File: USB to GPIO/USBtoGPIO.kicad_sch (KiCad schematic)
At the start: 3 parts, among them U1 STM32F030F4Px, U2 74HC595, U3 74HC165

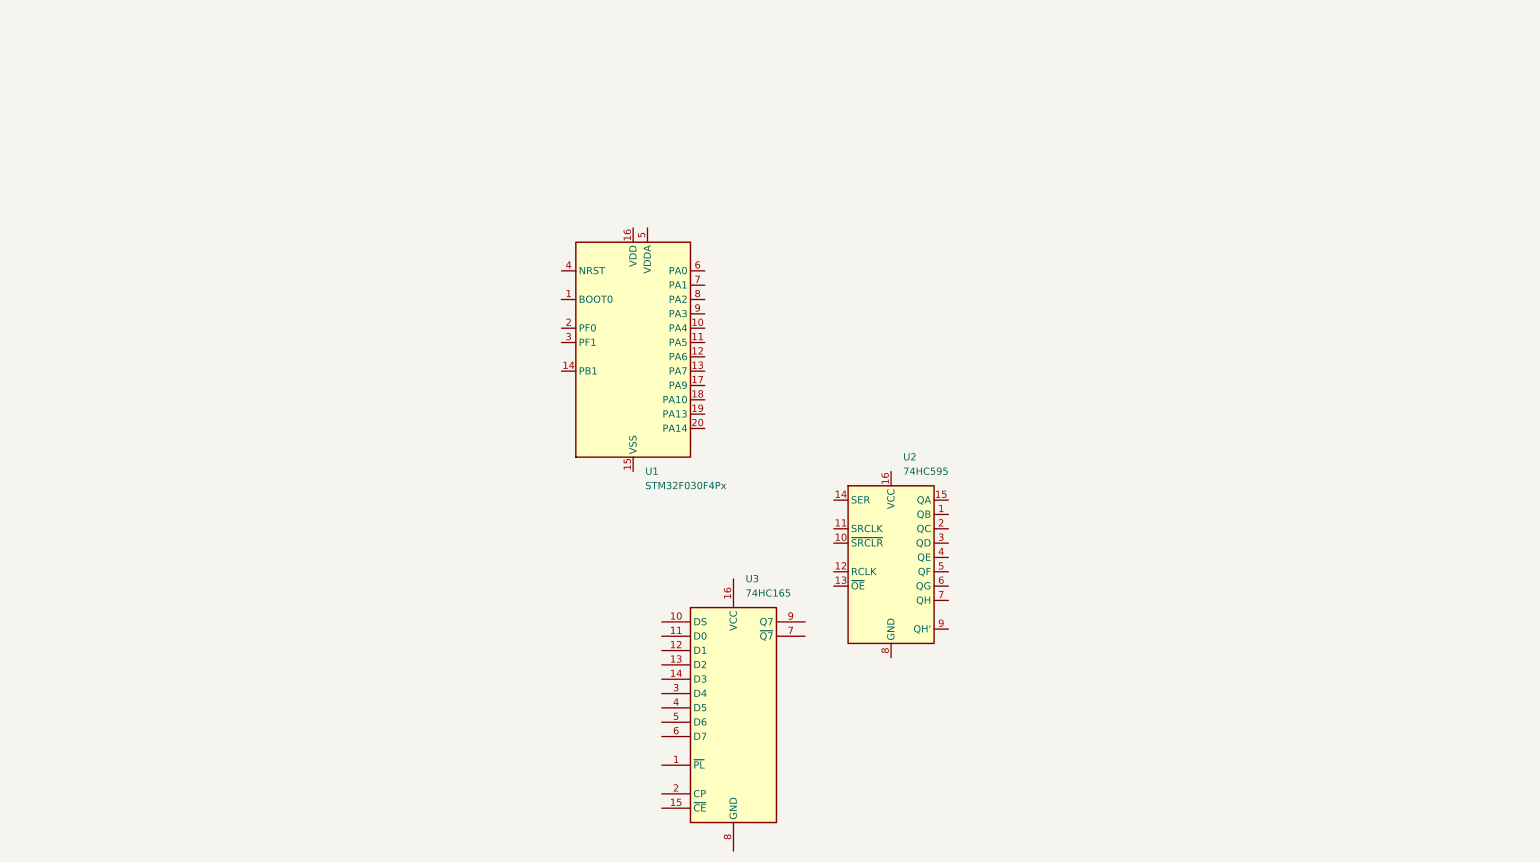
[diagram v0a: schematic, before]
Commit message: refresh
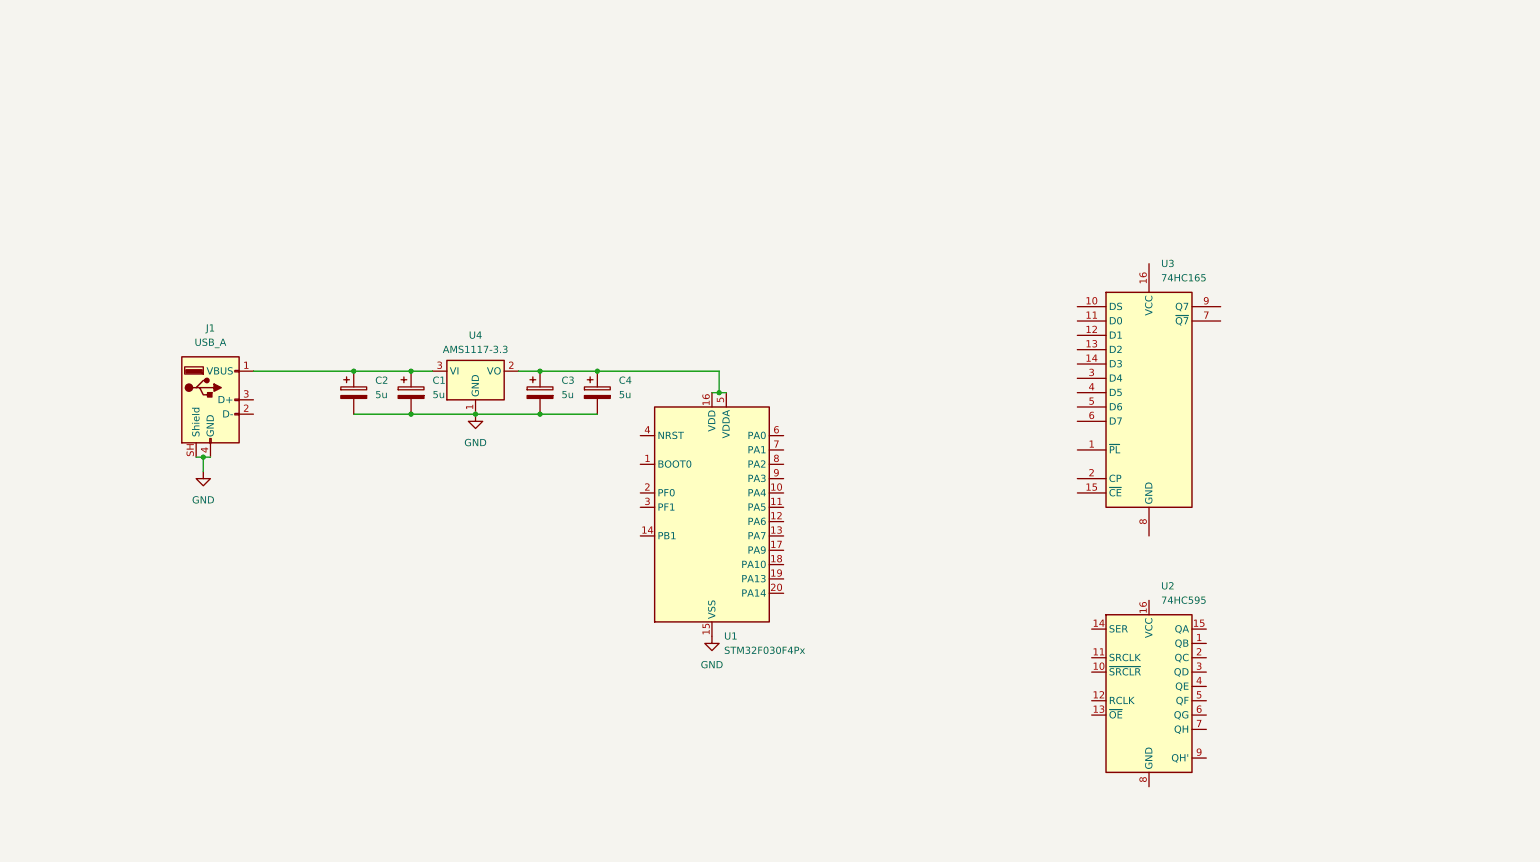
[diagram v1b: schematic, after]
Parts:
- added C1, C2, C3, C4: 5u, symbol Device:C_Polarized
- added J1: USB_A, Connector_USB:USB_A_TE_292303-7_Horizontal, symbol Connector:USB_A
- added U4: AMS1117-3.3, Package_TO_SOT_SMD:SOT-223-3_TabPin2, symbol Regulator_Linear:AMS1117-3.3
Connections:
- net GND: now reaches U1.15 (VSS)
- net GND: now also C1.2, C2.2, C3.2, C4.2, J1.4 (GND), J1.SH (Shield), U4.1 (GND)
- net at U1.16 (VDD): now also U1.5 (VDDA), C3.1, C4.1, U4.2 (VO)
- new net: C1.1, C2.1, J1.1 (VBUS), U4.3 (VI)
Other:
- moved on the sheet: U1, U2, U3

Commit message: refresh
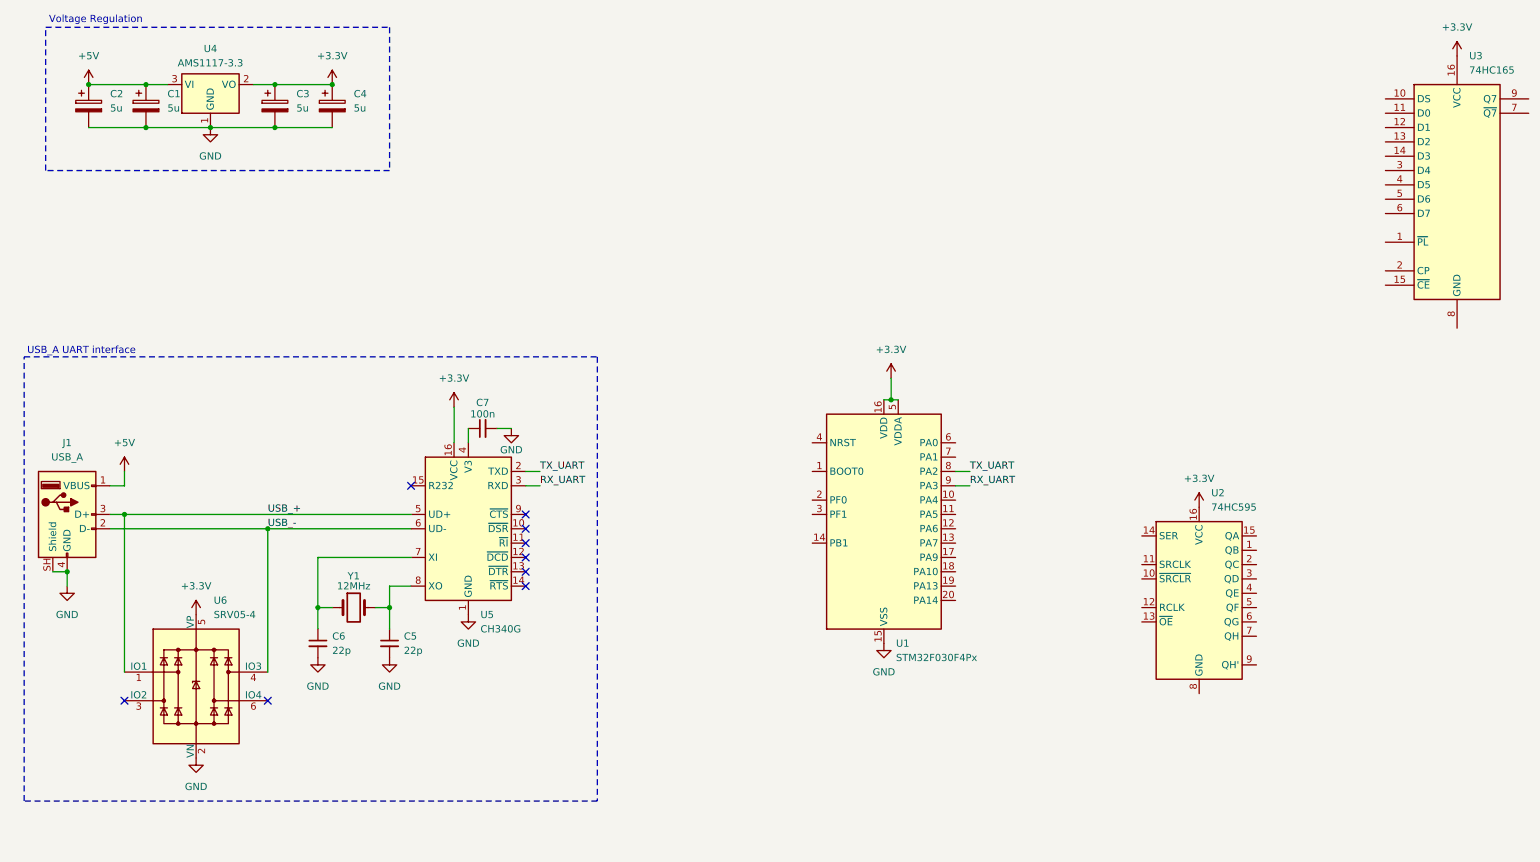
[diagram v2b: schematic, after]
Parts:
- added C5, C6: 22p, symbol Device:C_Small
- added C7: 100n, symbol Device:C_Small
- added U5: CH340G, Package_SO:SOIC-16_3.9x9.9mm_P1.27mm, symbol Interface_USB:CH340G
- added U6: SRV05-4, Package_TO_SOT_SMD:SOT-23-6, symbol Power_Protection:SRV05-4
- added Y1: 12MHz, symbol Device:Crystal
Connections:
- net GND: now also C5.2, C6.2, C7.2, U5.1 (GND), U6.2 (VN)
- net +5V: now reaches C1.1, C2.1, J1.1 (VBUS), U4.3 (VI)
- net +3.3V: now reaches C3.1, C4.1, U1.16 (VDD), U1.5 (VDDA), U4.2 (VO)
- net +3.3V: now also U2.16 (VCC), U3.16 (VCC), U5.16 (VCC), U6.5 (VP)
- net TX_UART: now reaches U1.8 (PA2)
- net TX_UART: now also U5.2 (TXD)
- net RX_UART: now reaches U1.9 (PA3)
- net RX_UART: now also U5.3 (RXD)
- net USB_-: now reaches J1.2 (D-)
- net USB_-: now also U5.6 (UD-), U6.4 (IO3)
- net USB_+: now reaches J1.3 (D+)
- net USB_+: now also U5.5 (UD+), U6.1 (IO1)
- new net: C6.1, U5.7 (XI), Y1.1
- new net: C5.1, U5.8 (XO), Y1.2
- new net: C7.1, U5.4 (V3)
- no-connect marks 0 -> 9
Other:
- note added: "USB_A UART interface"
- note added: "Voltage Regulation"
- moved on the sheet: C1, C2, C3, C4, J1, U1, U2, U3, U4

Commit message: refresh
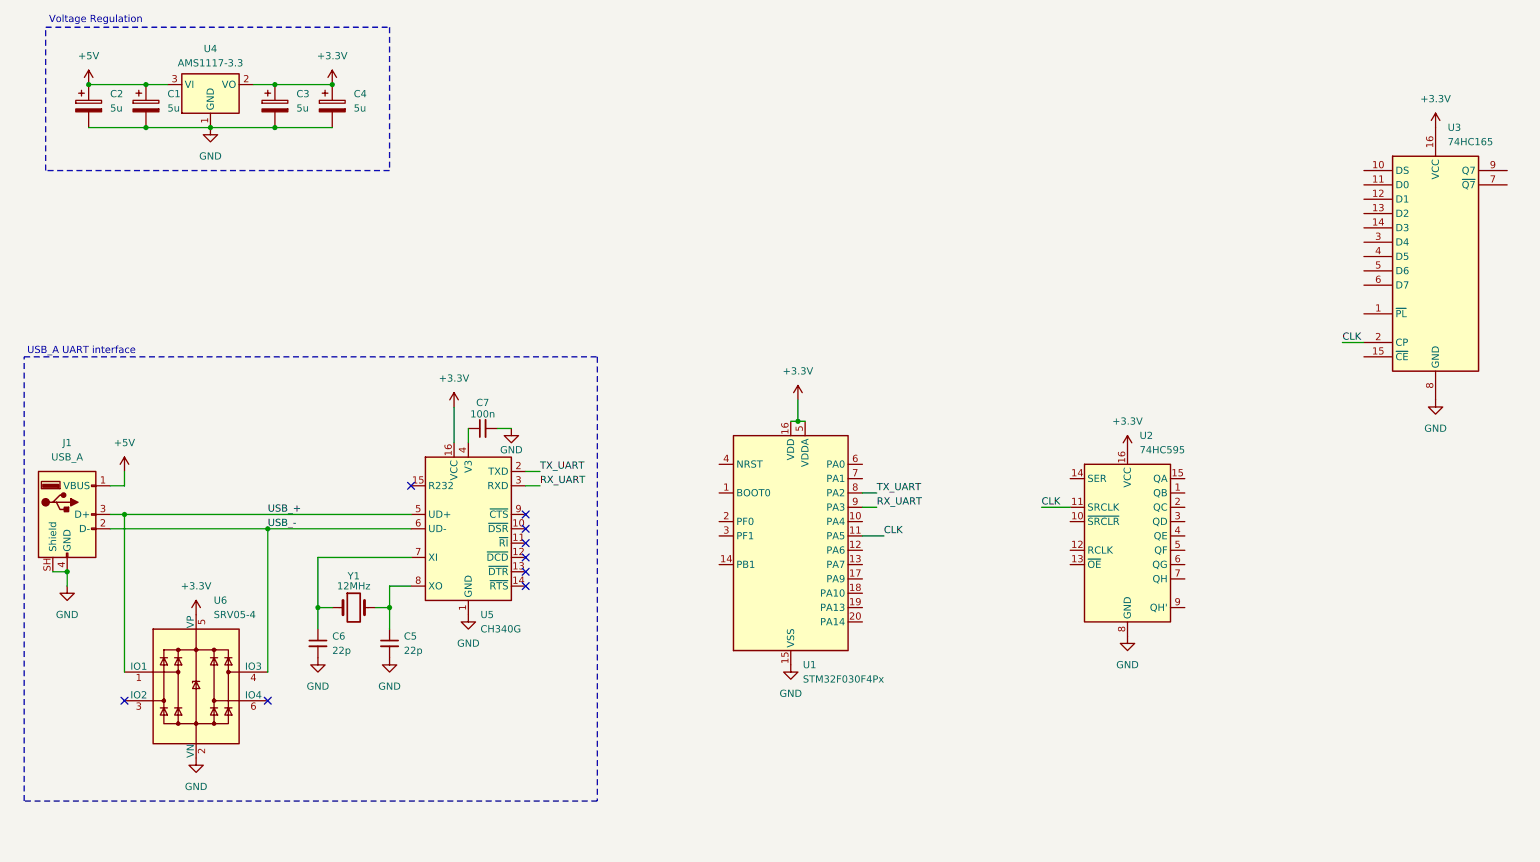
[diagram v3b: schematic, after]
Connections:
- net GND: now also U2.8 (GND), U3.8 (GND)
- net CLK: now reaches U1.11 (PA5)
- net CLK: now also U2.11 (SRCLK), U3.2 (CP)
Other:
- moved on the sheet: U1, U2, U3
